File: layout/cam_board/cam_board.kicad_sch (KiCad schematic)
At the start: 73 parts, among them J1 Debug, J2 USB Connector, J3 BATT_CONNECTOR, J4 LCD conn, J5 Stick conn, Q1 BSS138, SW1 BOOT0, SW2 NRST, SW3 USER, SW4 ON/OFF, U1 STM32F401CCUx, U2 USBLC6-2SC6, U4 AP2112K-3.3, U5 MCP73871-1AA, Y1 ECS-80-18-23B-JTN-TR, Y2 SC32S-7PF20PPM

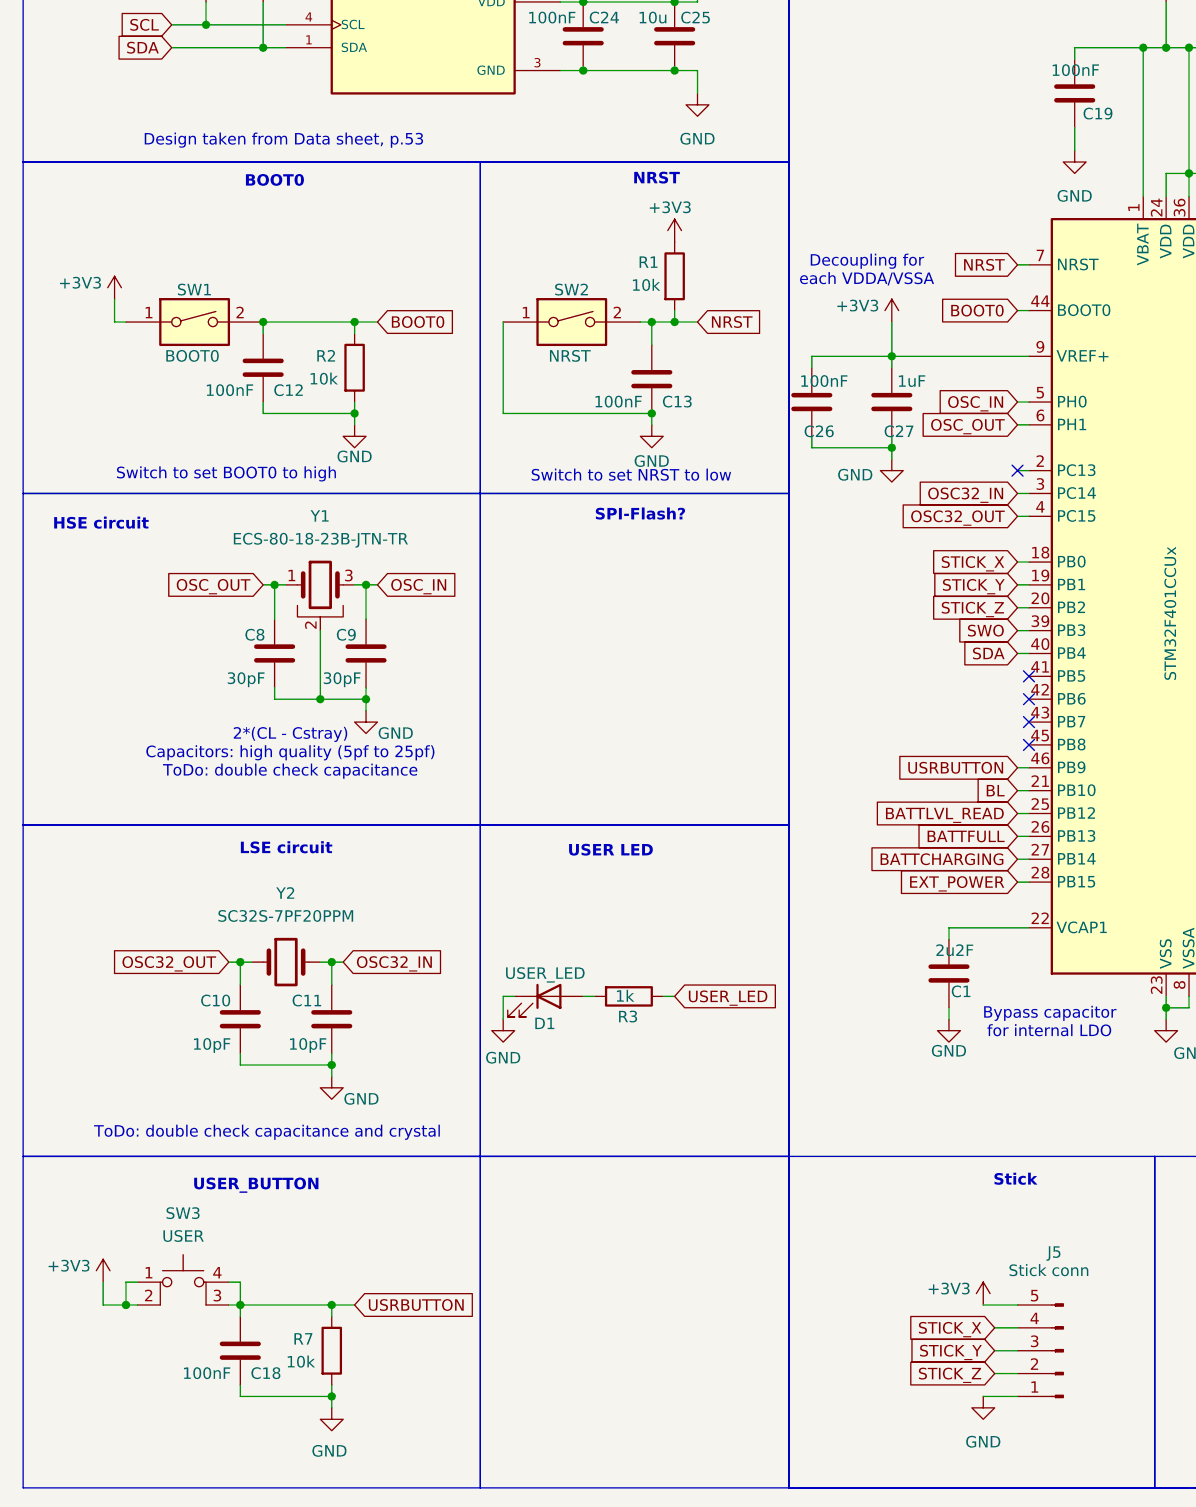
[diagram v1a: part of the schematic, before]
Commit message: Update layout and schematic
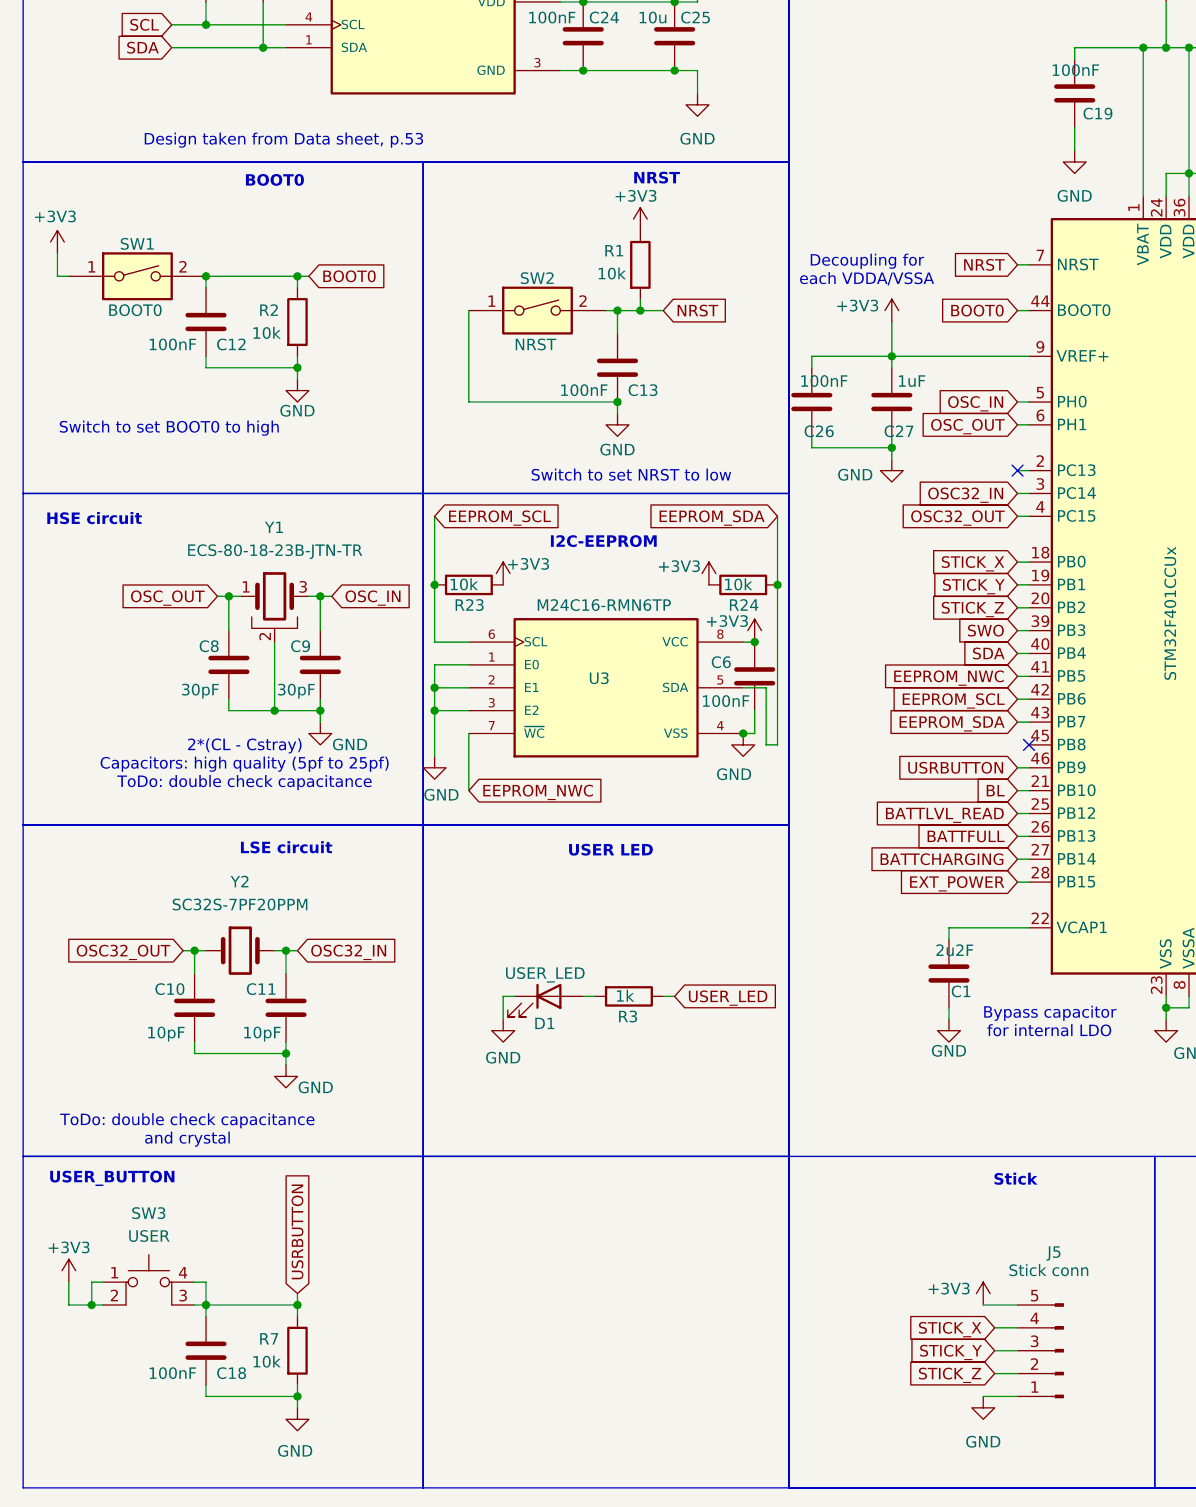
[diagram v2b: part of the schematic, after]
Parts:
- added C6: 100nF, Capacitor_SMD:C_0402_1005Metric_Pad0.74x0.62mm_HandSolder, symbol Device:C
- added R23, R24: 10k, Resistor_SMD:R_0603_1608Metric_Pad0.98x0.95mm_HandSolder, symbol Device:R
- added U3: M24C16-RMN6TP, A_Custom:SOIC127P600X175-8N, symbol Custom:M24C16-RMN6TP
- SW1, SW2, SW4: footprint Button_Switch_SMD:SW_DIP_SPSTx01_Slide_9.78x4.72mm_W8.61mm_P2.54mm -> Button_Switch_SMD:SW_DIP_SPSTx01_Slide_6.7x4.1mm_W8.61mm_P2.54mm_LowProfile
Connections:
- net +3V3: now also C6.2, R23.2, R24.1, U3.8 (VCC)
- net GND: now also C6.1, U3.1 (E0), U3.2 (E1), U3.3 (E2), U3.4 (VSS)
- net EEPROM_NWC: now reaches U1.41 (PB5)
- net EEPROM_NWC: now also U3.7 (~{WC})
- net EEPROM_SCL: now reaches U1.42 (PB6)
- net EEPROM_SCL: now also R23.1, U3.6 (SCL)
- net EEPROM_SDA: now reaches U1.43 (PB7)
- net EEPROM_SDA: now also R24.2, U3.5 (SDA)
- no-connect marks 8 -> 5
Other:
- note added: "I2C-EEPROM"
- note removed: "SPI-Flash?"
- moved on the sheet: C10, C11, C12, C13, C18, C8, C9, R1, R2, R7, SW1, SW2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

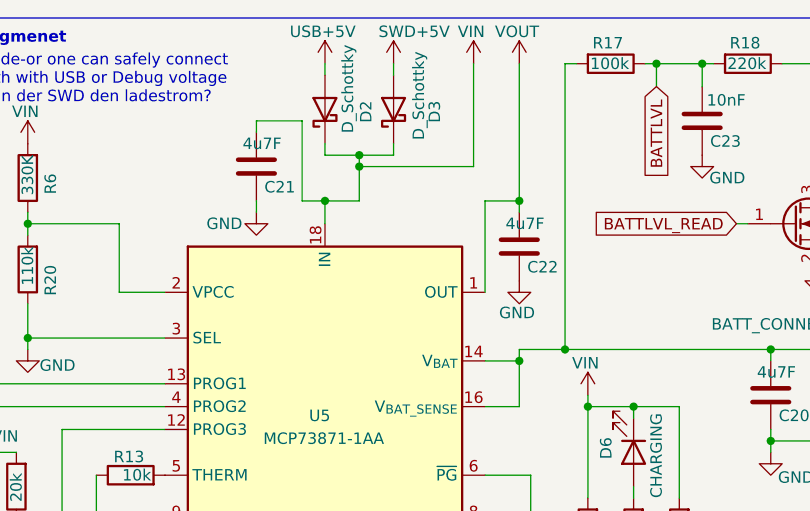
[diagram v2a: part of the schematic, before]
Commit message: Update layout and schematic
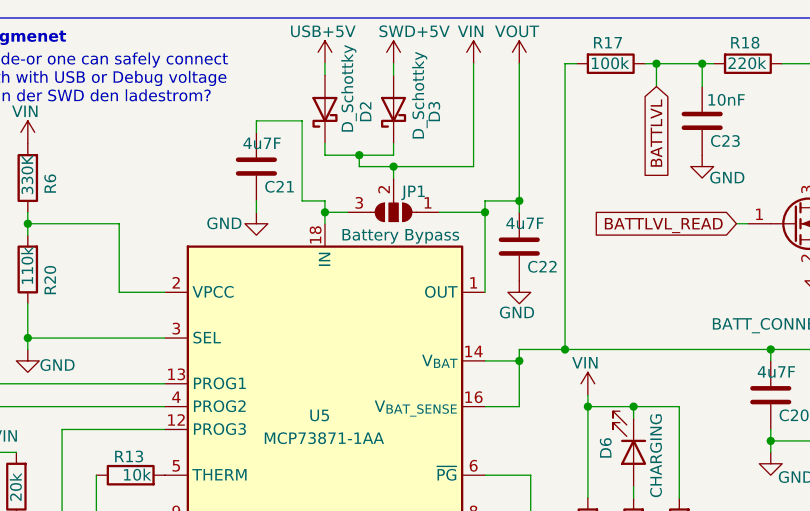
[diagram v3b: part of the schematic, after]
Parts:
- added JP1: Battery Bypass, Jumper:SolderJumper-3_P1.3mm_Open_RoundedPad1.0x1.5mm_NumberLabels, symbol Jumper:SolderJumper_3_Open
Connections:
- net VIN: now also JP1.2 (C); no longer C21.2, U5.18 (IN), U5.19 (IN)
- net VOUT: now also JP1.1 (A)
- new net: C21.2, JP1.3 (B), U5.18 (IN), U5.19 (IN)
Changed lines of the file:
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@@
 	)
 	(junction
-		(at 220.98 33.02)
-		(diameter 0)
-		(color 0 0 0 0)
-	)
-	(junction
 		(at 137.16 35.56)
 		(diameter 0)
@@
 	)
 	(junction
+		(at 220.98 34.29)
+		(diameter 0)
+		(color 0 0 0 0)
+	)
+	(junction
 		(at 187.96 35.56)
 		(diameter 0)
@@
 	)
 	(junction
-		(at 224.79 29.21)
+		(at 43.18 185.42)
 		(diameter 0)
 		(color 0 0 0 0)
 	)
 	(junction
-		(at 43.18 185.42)
+		(at 190.5 81.28)
 		(diameter 0)
 		(color 0 0 0 0)
 	)
 	(junction
-		(at 190.5 81.28)
+		(at 228.6 29.21)
 		(diameter 0)
 		(color 0 0 0 0)
@@
 	)
 	(junction
+		(at 238.76 34.29)
+		(diameter 0)
+		(color 0 0 0 0)
+	)
+	(junction
 		(at 270.51 59.69)
 		(diameter 0)
@@
 	(wire
 		(pts
-			(xy 238.76 33.02) (xy 238.76 43.18)
+			(xy 238.76 33.02) (xy 238.76 34.29)
 		)
 		(stroke
@@
 	(wire
 		(pts
+			(xy 220.98 34.29) (xy 220.98 35.56)
+		)
+		(stroke
+			(width 0)
+			(type default)
+		)
+	)
+	(wire
+		(pts
 			(xy 43.18 184.15) (xy 43.18 185.42)
 		)
@@
 	(wire
 		(pts
-			(xy 224.79 29.21) (xy 237.49 29.21)
+			(xy 224.79 29.21) (xy 228.6 29.21)
 		)
 		(stroke
@@
 	(wire
 		(pts
-			(xy 220.98 33.02) (xy 220.98 35.56)
+			(xy 220.98 33.02) (xy 220.98 34.29)
 		)
 		(stroke
@@
 	(wire
 		(pts
-			(xy 220.98 33.02) (xy 224.79 33.02)
-		)
-		(stroke
-			(width 0)
-			(type default)
-		)
-	)
-	(wire
-		(pts
 			(xy 209.55 118.11) (xy 209.55 123.19)
 		)
@@
 	(wire
 		(pts
+			(xy 233.68 34.29) (xy 238.76 34.29)
+		)
+		(stroke
+			(width 0)
+			(type default)
+		)
+	)
+	(wire
+		(pts
 			(xy 158.75 45.72) (xy 158.75 44.45)
 		)
@@
 	(wire
 		(pts
+			(xy 238.76 34.29) (xy 238.76 43.18)
+		)
+		(stroke
+			(width 0)
+			(type default)
+		)
+	)
+	(wire
+		(pts
 			(xy 250.19 73.66) (xy 250.19 74.93)
 		)
@@
 	(wire
 		(pts
+			(xy 228.6 29.21) (xy 228.6 30.48)
+		)
+		(stroke
+			(width 0)
+			(type default)
+		)
+	)
+	(wire
+		(pts
 			(xy 43.18 173.99) (xy 43.18 175.26)
 		)
@@
 	(wire
 		(pts
+			(xy 228.6 29.21) (xy 237.49 29.21)
+		)
+		(stroke
+			(width 0)
+			(type default)
+		)
+	)
+	(wire
+		(pts
 			(xy 190.5 81.28) (xy 190.5 83.82)
 		)
@@
 	(wire
 		(pts
+			(xy 220.98 34.29) (xy 223.52 34.29)
+		)
+		(stroke
+			(width 0)
+			(type default)
+		)
+	)
+	(wire
+		(pts
 			(xy 151.13 173.99) (xy 153.67 173.99)
 		)
@@
 	(wire
 		(pts
-			(xy 224.79 29.21) (xy 224.79 33.02)
-		)
-		(stroke
-			(width 0)
-			(type default)
-		)
-	)
-	(wire
-		(pts
 			(xy 218.44 24.13) (xy 213.36 24.13)
 		)
@@
 					(unit 1)
 				)
+			)
+		)
+	)
+	(symbol
+		(lib_id "Jumper:SolderJumper_3_Open")
+		(at 228.6 34.29 180)
+		(unit 1)
+		(exclude_from_sim no)
+		(in_bom no)
+		(on_board yes)
+		(dnp no)
+		(property "Reference" "JP1"
+			(at 230.886 32.004 0)
+			(effects
+				(font
+					(size 1.27 1.27)
+				)
+			)
+		)
+		(property "Value" "Battery Bypass"
+			(at 229.362 36.83 0)
+			(effects
+				(font
+					(size 1.27 1.27)
+				)
+			)
+		)
+		(property "Footprint" "Jumper:SolderJumper-3_P1.3mm_Open_RoundedPad1.0x1.5mm_NumberLabels"
+			(at 228.6 34.29 0)
+			(effects
+				(font
+					(size 1.27 1.27)
+				)
+				(hide yes)
+			)
+		)
+		(property "Datasheet" "~"
+			(at 228.6 34.29 0)
+			(effects
+				(font
+					(size 1.27 1.27)
+				)
+				(hide yes)
+			)
+		)
+		(property "Description" "Solder Jumper, 3-pole, open"
+			(at 228.6 34.29 0)
+			(effects
+				(font
+					(size 1.27 1.27)
+				)
+				(hide yes)
+			)
+		)
+		(pin "3"
+		)
+		(pin "2"
+		)
+		(pin "1"
+		)
+		(instances
+			(project "cam_board"
+				(path "/eee23683-93c4-45fa-9c00-e358d0d25f58"
+					(reference "JP1")
+					(unit 1)
+				)
